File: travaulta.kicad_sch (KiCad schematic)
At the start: 33 parts, among them J1 USB_C_Receptacle_USB2.0, J2 JST, Q1 2N7002, SW38 SW_MEC_5G, U1 STM32F411CCUx, U2 XC6206PxxxMR, Y1 16 MHz

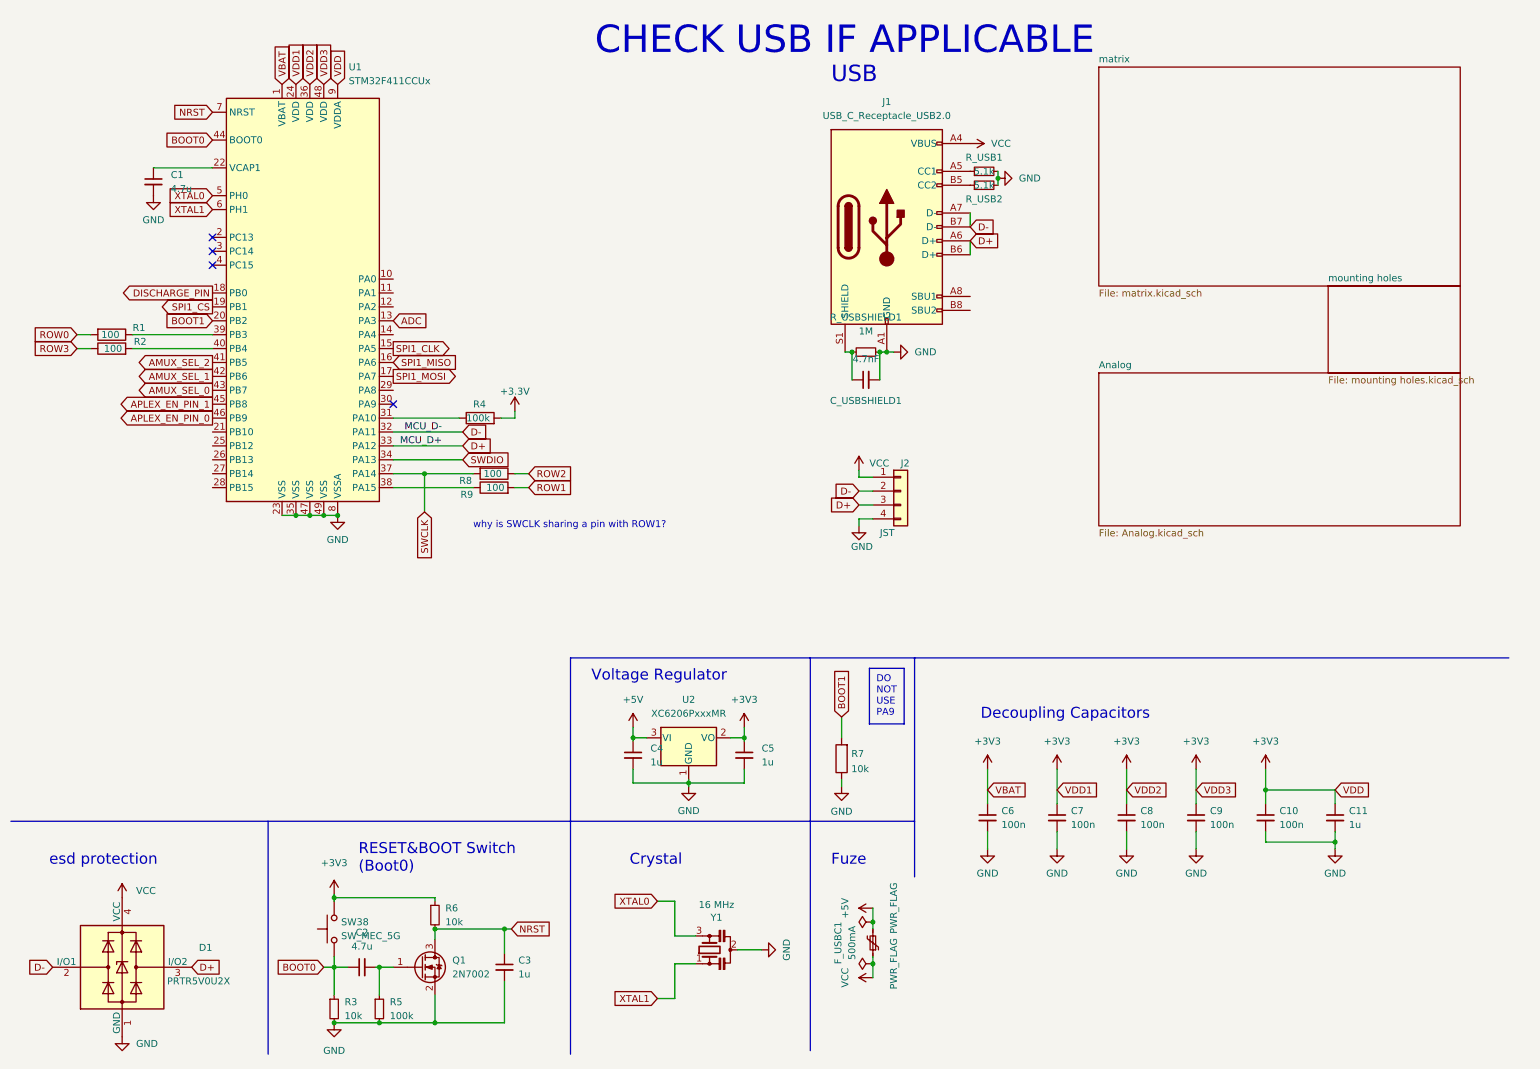
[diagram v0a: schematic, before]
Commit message: early routing
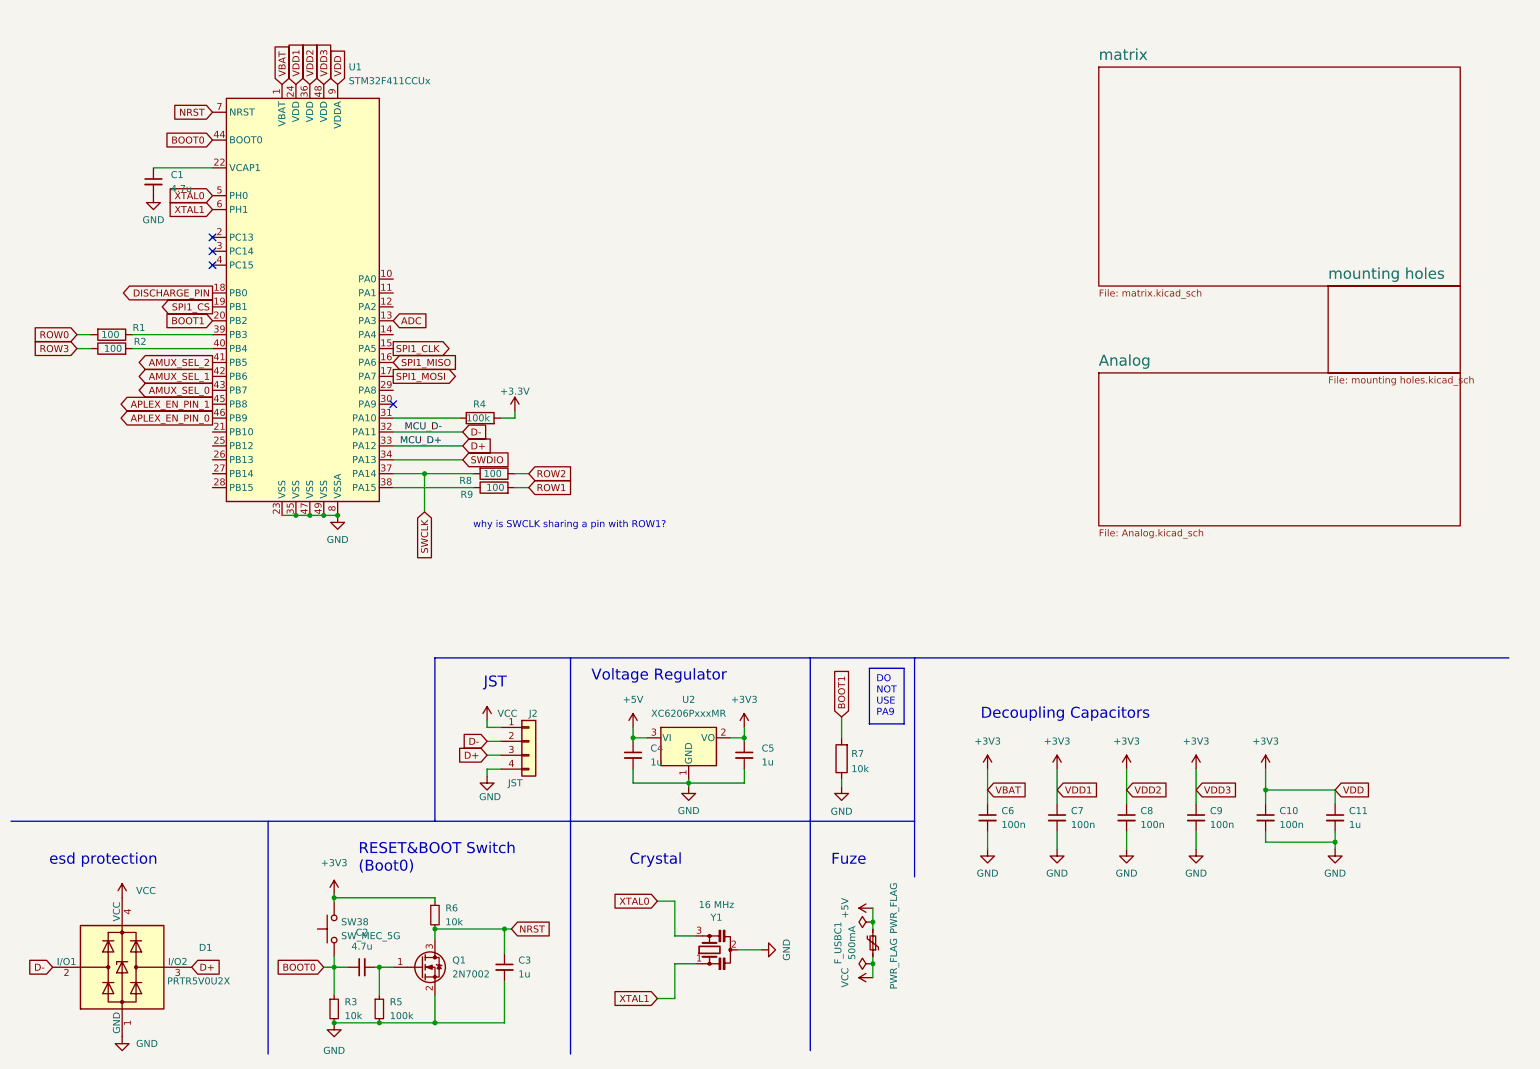
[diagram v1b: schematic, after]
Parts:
- removed C_USBSHIELD1: 4.7nF, Capacitor_SMD:C_0402_1005Metric, symbol Device:C_Small
- removed J1: USB_C_Receptacle_USB2.0, Connector_USB:USB_C_Receptacle_HRO_TYPE-C-31-M-12, symbol Connector:USB_C_Receptacle_USB2.0
- removed R_USB1, R_USB2: 5.1k, Resistor_SMD:R_0402_1005Metric, symbol Device:R_Small
- removed R_USBSHIELD1: 1M, Resistor_SMD:R_0402_1005Metric, symbol Device:R_Small
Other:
- note added: "JST"
- note removed: "CHECK USB IF APPLICABLE"
- note removed: "USB"
- moved on the sheet: J2
